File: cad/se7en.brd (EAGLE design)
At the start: 64.1 x 34 mm, 67 parts, among them CN1 MICROSD-EJECT, CN3 DO NOT PLACE, CN4 DO NOT PLACE, CN5 DO NOT PLACE, CN6 DO NOT PLACE, CN7 DO NOT PLACE, Q1 FDC6329S, SW1 SWITCHKMR211, SW2 SWITCHKMR211, U1 ATSAME70, U2 MCP73831/OT, X1 12MHz, X2 32k768

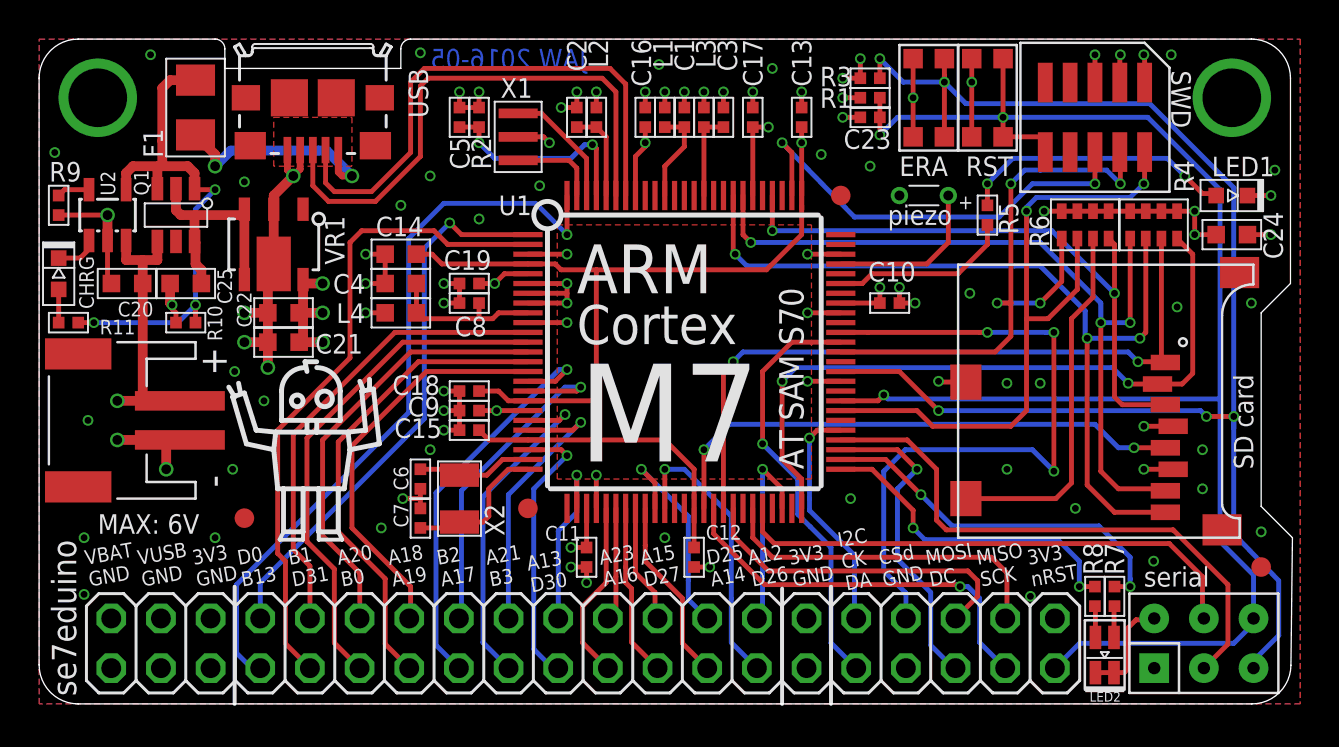
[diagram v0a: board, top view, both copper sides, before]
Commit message: tweak
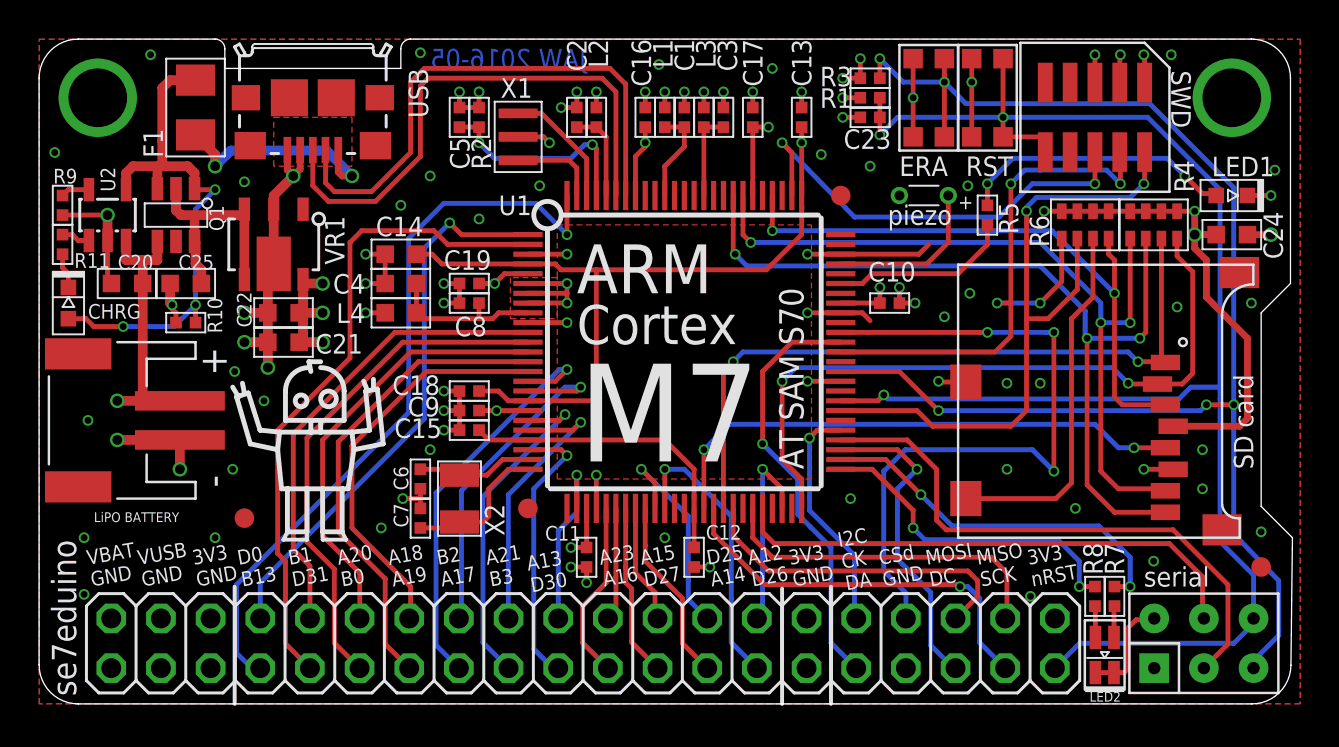
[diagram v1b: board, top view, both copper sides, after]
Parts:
- moved R11 4.01 mm to (57.2, 58.5), turned to 270 degrees
- moved LED3 1.58 mm to (57.5, 55.5)
- moved R9 0.20 mm to (57.2, 60.5)
- moved U$3 0.20 mm to (70.1, 47.8)
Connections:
- removed net PINA22: U1.26
- net N$10: now also R11.1; no longer LED3.C
- net N$12: now also LED3.C, R11.2; no longer LED3.A, R11.1
- net VIN: now also LED3.A; no longer R11.2
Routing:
- net VCC: track 45.2 -> 58.2 mm, vias 18 -> 17
- net GND: track 93.2 -> 99.3 mm, vias 86 -> 88
- net VBAT: track 32.7 -> 30.5 mm
- net VIN: track 27.1 -> 27.9 mm
- net N$10: track 2.19 -> 1.47 mm
- net ERASE: track 73.8 -> 74.4 mm
- added copper zone on layer 1, net N$18
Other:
- board text added: "LiPO BATTERY"
- board text removed: "MAX: 6V"
